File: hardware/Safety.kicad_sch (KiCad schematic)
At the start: 17 parts, among them K2 PB134024, Q1 2N7002, Q2 2N7002, Q3 2N7002, U2 74LVC1G86, U3 74AUP1G32

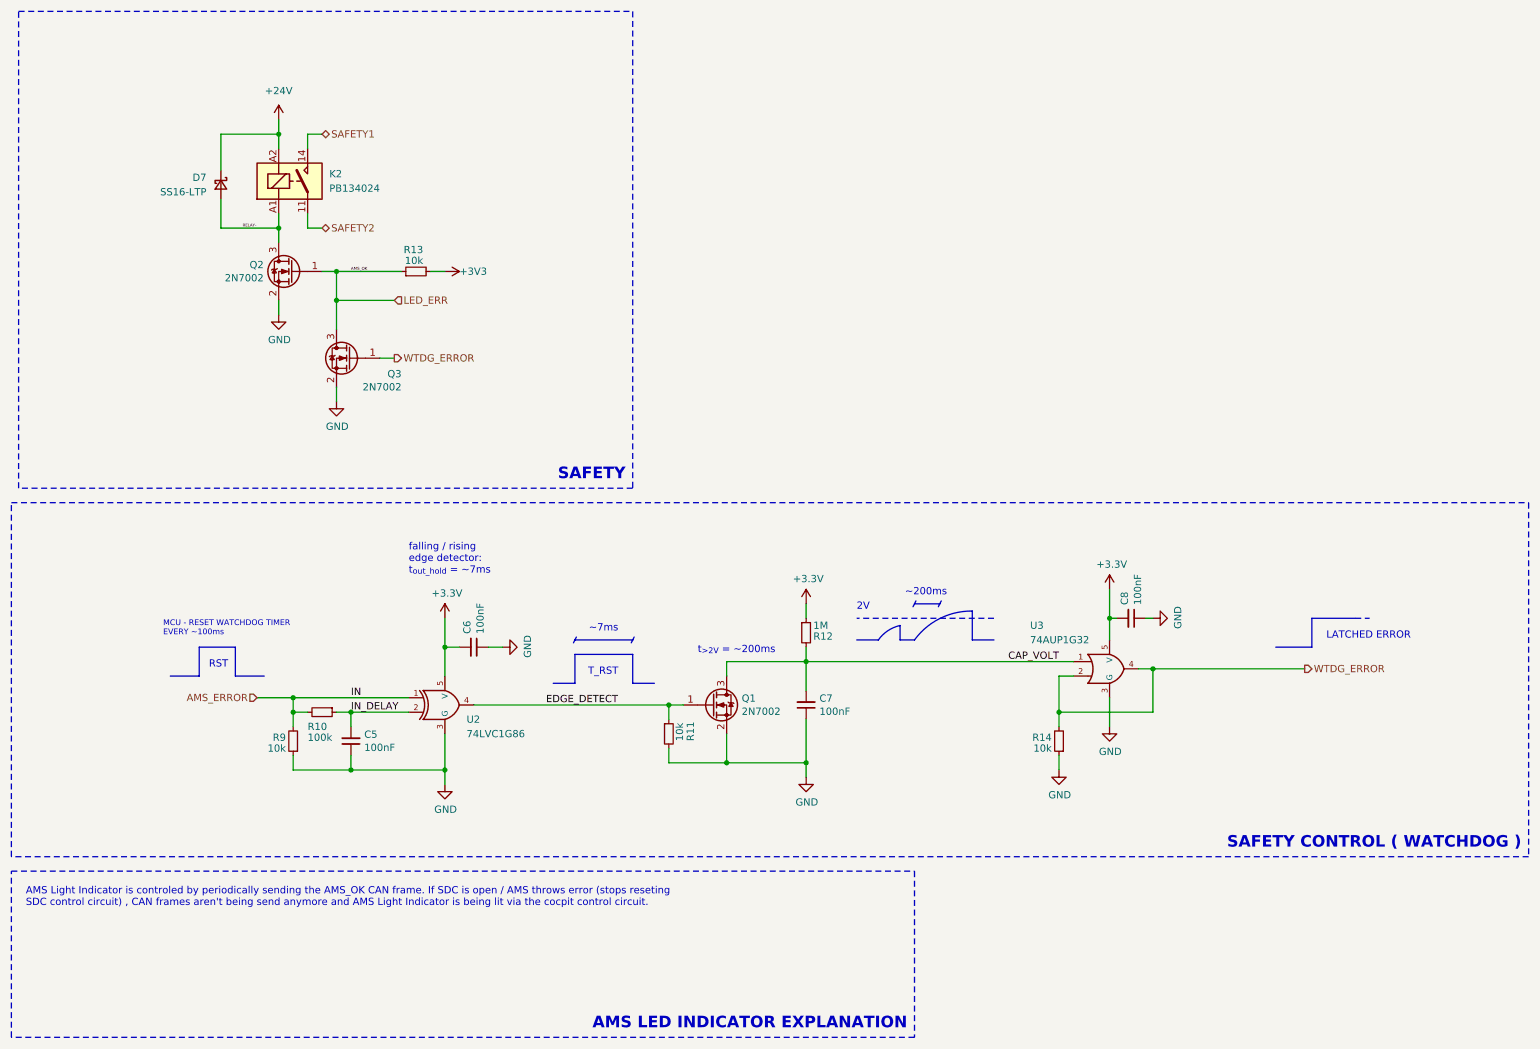
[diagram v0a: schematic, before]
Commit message: mama comit
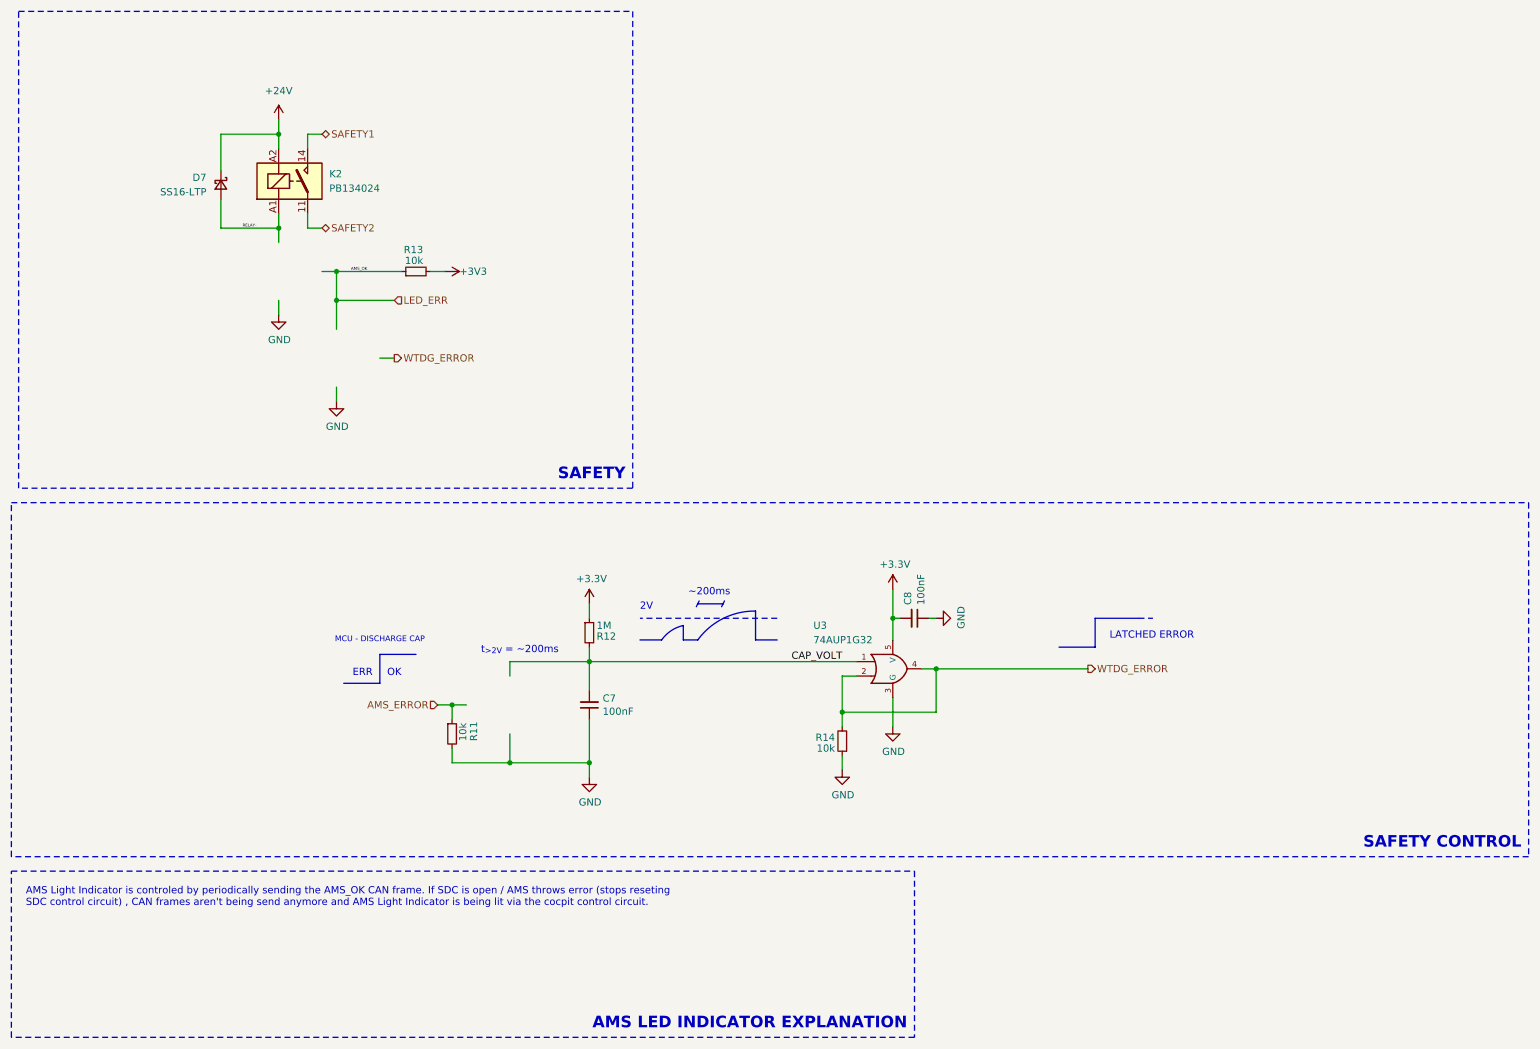
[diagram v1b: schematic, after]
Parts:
- removed C5, C6: 100nF, Capacitor_SMD:C_0603_1608Metric, symbol Device:C_Small
- removed Q1, Q2, Q3: 2N7002, Package_TO_SOT_SMD:SOT-23, symbol Transistor_FET:2N7002
- removed R10: 100k, Resistor_SMD:R_0603_1608Metric, symbol Device:R_Small
- removed R9: 10k, Resistor_SMD:R_0603_1608Metric, symbol Device:R_Small
- removed U2: 74LVC1G86, Package_TO_SOT_SMD:SOT-23-5, symbol 74xGxx:74LVC1G86
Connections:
- net EDGE_DETECT is gone; now on net AMS_ERROR: R11.1
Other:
- note added: "ERR"
- note added: "MCU - DISCHARGE CAP"
- note added: "OK"
- note added: "SAFETY CONTROL"
- note removed: "MCU - RESET WATCHDOG TIMER EVERY ~100ms"
- note removed: "RST"
- note removed: "SAFETY CONTROL ( WATCHDOG )"
- note removed: "T_RST"
- note removed: "falling / rising edge detector: t_{out_hold} = ~7ms"
- note removed: "~7ms"
- moved on the sheet: C7, C8, R11, R12, R14, U3
